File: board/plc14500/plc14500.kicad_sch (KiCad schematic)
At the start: 8 parts

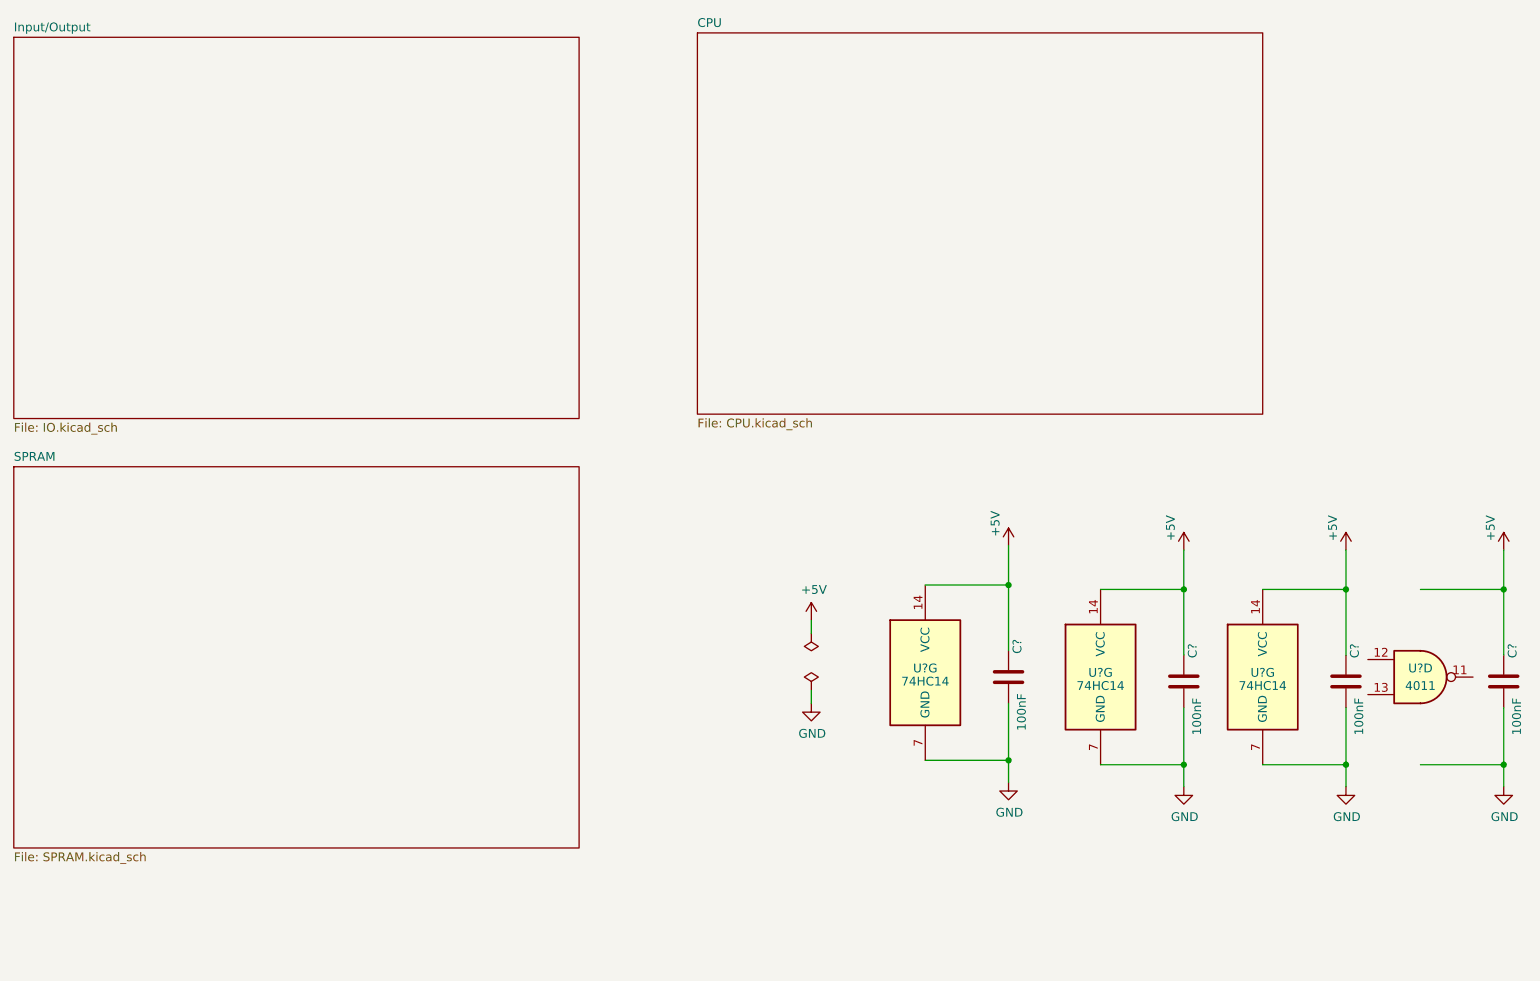
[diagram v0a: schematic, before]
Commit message: Feature/rev.d (#19)
* First tests for a rust upload tool, WIP

* Rearrange LEDs

* Remove kicad backups

* REV.D Schema updates

* Restore PCB anchoring holes

* Address ERC errors

* Cleanup, ready to route

* REV.D first proto

* Fix issues on REV.D0

* REV.D schema fixes, better assembler output, some docs

* Add ignore of kicad lock files

* Fixes

* route

* Re-route REV.D, fab files next round

* Re-route REV.D, fab files next round

* Rev.d

* Added reset cap from program line

* REV.D artifacts

* Cleanup REV.D

* Remove old file
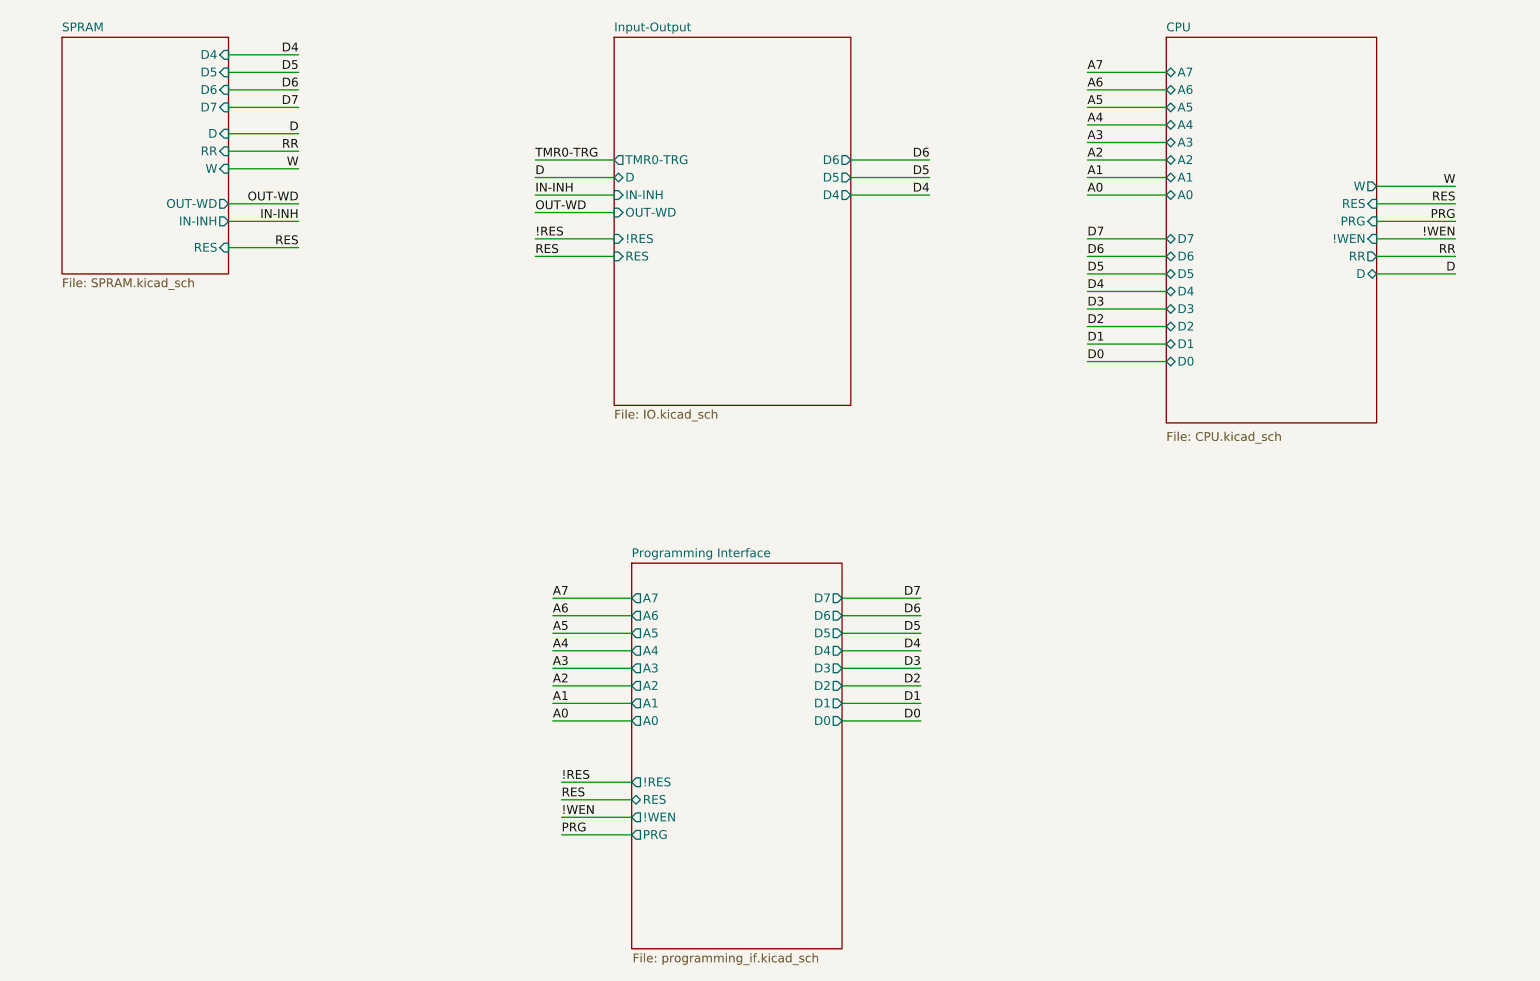
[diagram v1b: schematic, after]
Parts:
- removed C? (x4): 100nF, Capacitor_THT:C_Rect_L7.2mm_W2.5mm_P5.00mm_FKS2_FKP2_MKS2_MKP2, symbol Device:C
- removed U? (x3): 74HC14, Package_DIP:DIP-14_W7.62mm_LongPads, symbol 74xx:74HC14
- removed U?: 4011, Package_DIP:DIP-14_W7.62mm_LongPads, symbol 4xxx:4011
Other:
- sheet Input/Output renamed Input-Output
- added sheet Programming Interface (programming_if.kicad_sch)
- sheet CPU ports: added !WEN, A0, A1, A2, A3, A4, A5, A6, A7, D, D0, D1, D2, D3, D4, D5, D6, D7, PRG, RES, RR, W; removed none
- sheet Input-Output ports: added !RES, D, D4, D5, D6, IN-INH, OUT-WD, RES, TMR0-TRG; removed none
- sheet SPRAM ports: added D, D4, D5, D6, D7, IN-INH, OUT-WD, RES, RR, W; removed none
